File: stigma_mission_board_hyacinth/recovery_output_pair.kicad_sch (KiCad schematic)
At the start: 17 parts, among them J10 43045-0400, Q10 TPH4R008NH, Q12 TPH4R008NH, U14 TF0216, U17 TF0216

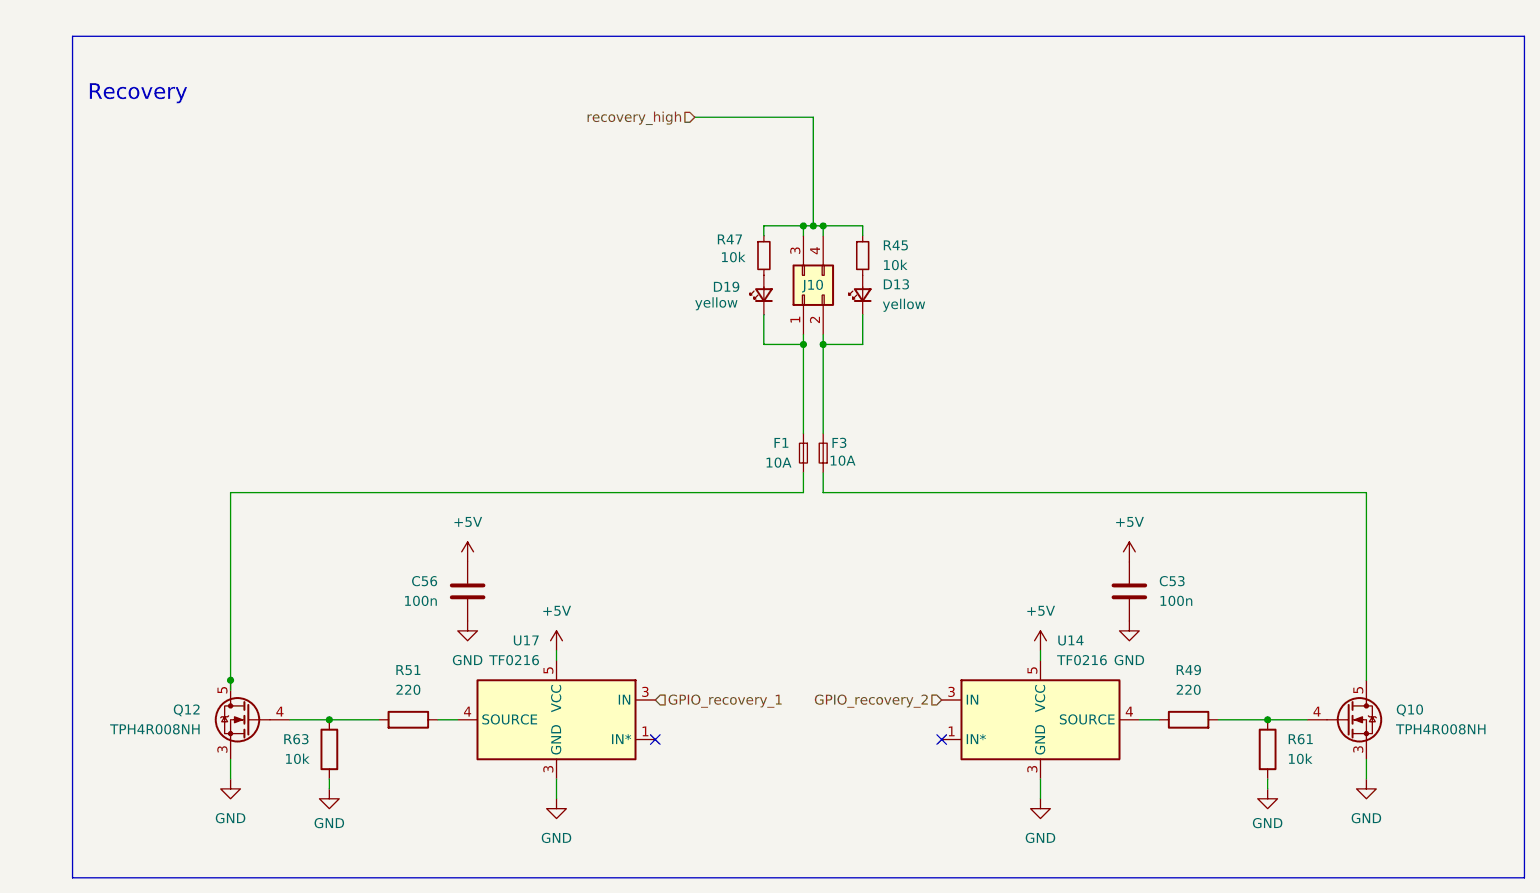
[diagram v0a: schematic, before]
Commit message: start routing
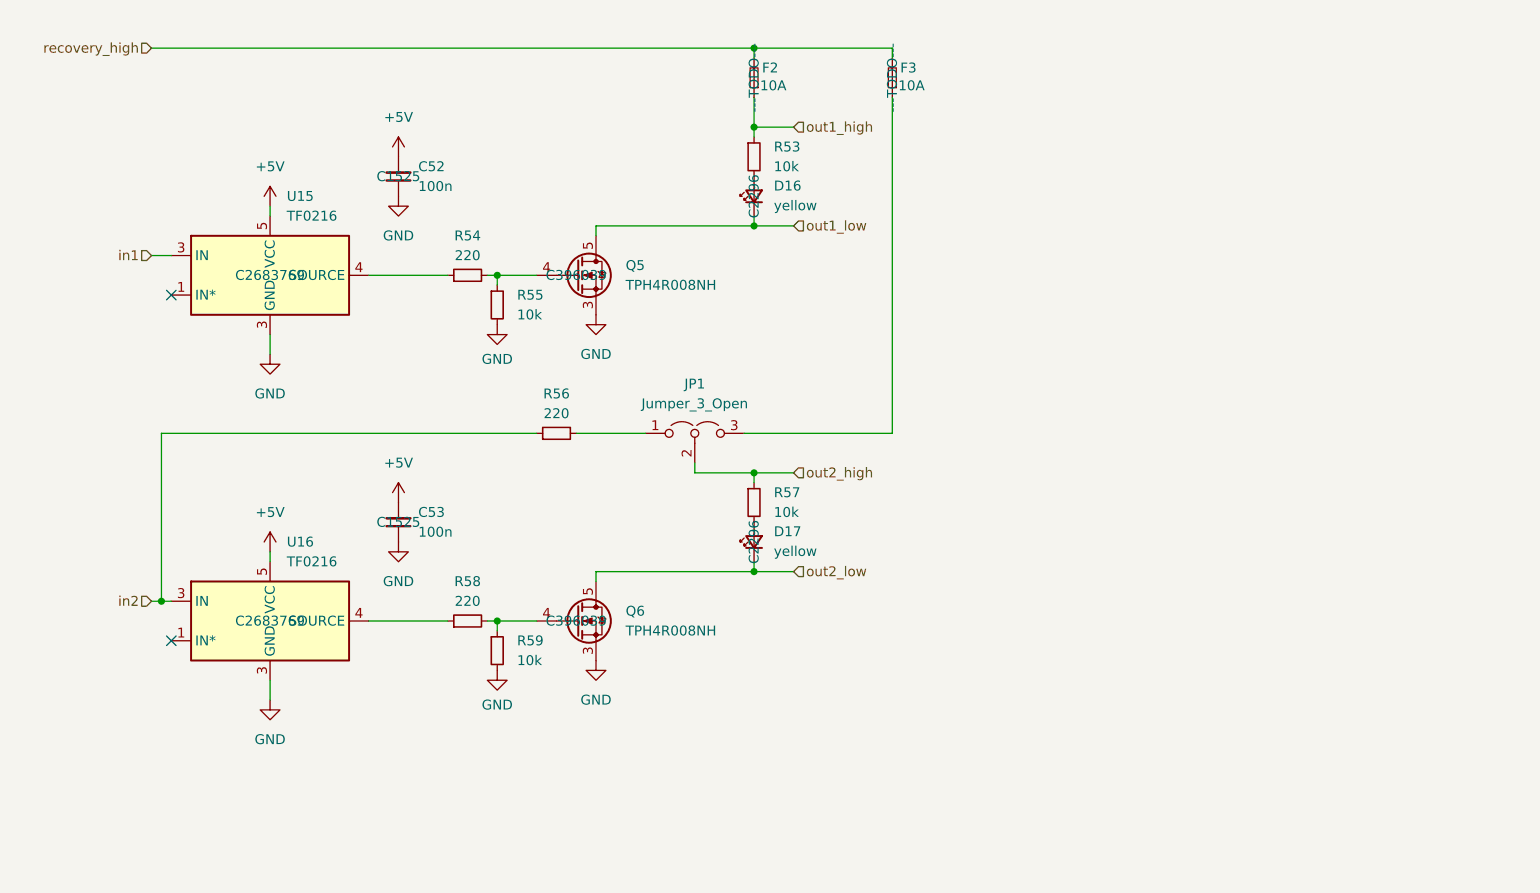
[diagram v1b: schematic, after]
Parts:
- removed C53, C56: 100n, Capacitor_SMD:C_0603_1608Metric, symbol Device:C
- removed D13, D19: yellow, symbol Device:LED_Small
- removed F1: 10A, Fuse:Fuse_1206_3216Metric, symbol Device:Fuse_Small
- removed J10: 43045-0400, stigma:Molex_Micro-Fit_3.0_43045-0400_2x02_P3.00mm_Horizontal, symbol Connector_Generic:Conn_02x02_Top_Bottom
- removed Q10, Q12: TPH4R008NH, Package_SO:SSOP-8_5.25x5.24mm_P1.27mm, symbol Transistor_FET:DMG2302U
- removed R45, R47: 10k, symbol Device:R_Small
- removed R49, R51: 220, symbol Device:R
- removed R61, R63: 10k, Resistor_SMD:R_0603_1608Metric, symbol Device:R
- removed U14, U17: TF0216, Package_TO_SOT_SMD:SOT-23-5, symbol Driver_FET:ZXGD3003E6
- added C52, C53: 100n, Capacitor_SMD:C_0402_1005Metric, symbol Device:C_Small
- added D16, D17: yellow, LED_SMD:LED_0603_1608Metric, symbol Device:LED_Small
- added F2: 10A, Fuse:Fuse_1206_3216Metric, symbol Device:Fuse_Small
- added JP1: Jumper_3_Open, Connector_PinHeader_2.54mm:PinHeader_1x03_P2.54mm_Vertical, symbol Jumper:Jumper_3_Open
- added Q5, Q6: TPH4R008NH, Package_SO:SSOP-8_5.25x5.24mm_P1.27mm, symbol Transistor_FET:DMG2302U
- added R53, R55, R57, R59: 10k, Resistor_SMD:R_0402_1005Metric, symbol Device:R_Small
- added R54, R56, R58: 220, Resistor_SMD:R_0402_1005Metric, symbol Device:R_Small
- added U15, U16: TF0216, Package_TO_SOT_SMD:SOT-23-5, symbol Driver_FET:ZXGD3003E6
- F3: LCSC (none) -> ---TODO---
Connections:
- net +5V: now also C52.2, C53.2, U15.5 (VCC), U16.5 (VCC)
- net GND: now also C52.1, C53.1, Q5.3 (S), Q6.3 (S), R55.2, R59.2, U15.3 (GND), U16.3 (GND)
- net recovery_high: now also F3.2, F2.2
- net at F3.1: now also JP1.3 (B)
- new net: R58.1, U16.4 (SOURCE)
- new net: Q6.4 (G), R58.2, R59.1
- new net: Q5.4 (G), R54.2, R55.1
- new net: D17.2 (A), R57.2
- new net: R54.1, U15.4 (SOURCE)
- new net: JP1.1 (A), R56.2
- new net: D16.2 (A), R53.2
- new net in1: U15.3 (GND)
- new net in2: R56.1, U16.3 (GND)
- new net out1_high: F2.1, R53.1
- new net out1_low: D16.1 (K), Q5.5 (D)
- new net out2_high: JP1.2 (C), R57.1
- new net out2_low: D17.1 (K), Q6.5 (D)
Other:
- note removed: "Recovery"
- title: Recovery Output -> (none)
